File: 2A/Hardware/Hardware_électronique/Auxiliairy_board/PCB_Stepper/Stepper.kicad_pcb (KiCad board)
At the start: 2 copper layers, 35 x 30 mm, 45 parts, among them J1 UART_IN, J2 Conn_ST_STDC14, J3 Conn_01x03_Pin, J4 Conn_01x03_Pin, U4 AZ1117-3.3, U5 STM32G071CBUx

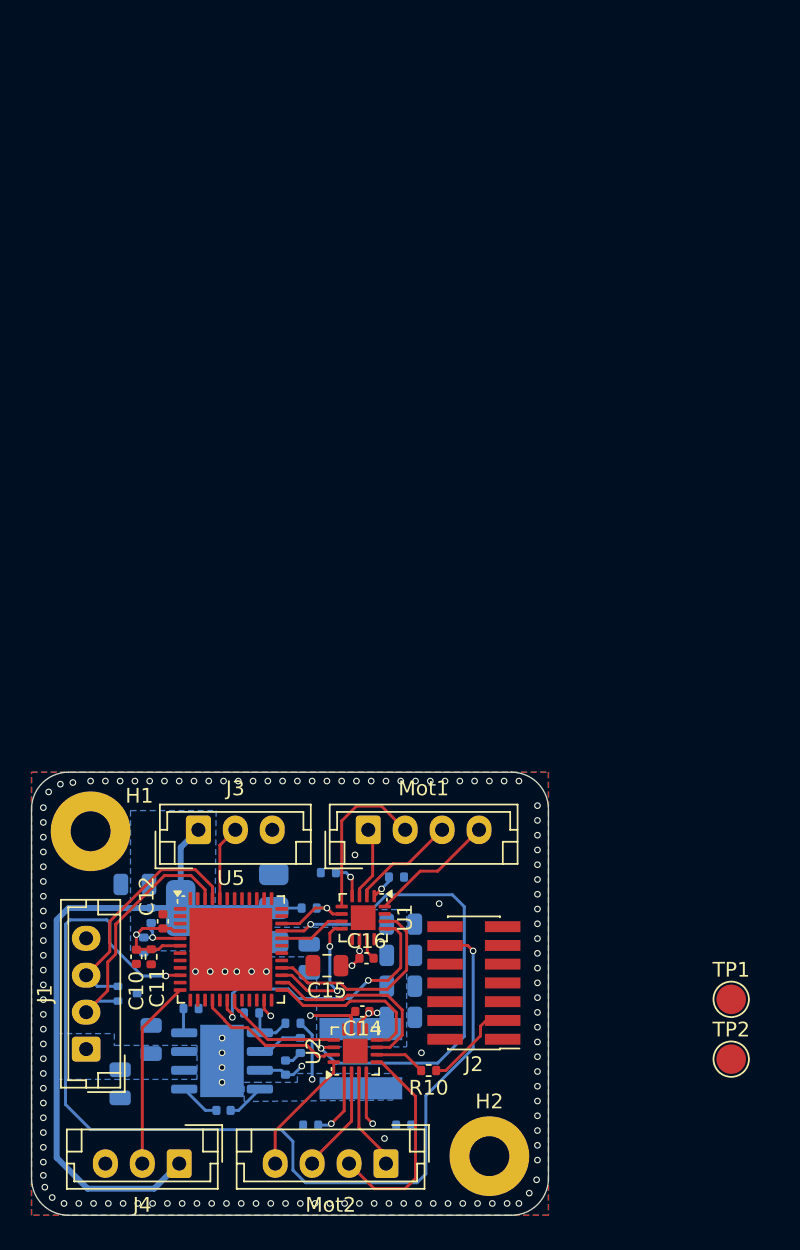
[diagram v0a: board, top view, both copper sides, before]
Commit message: recommit to be sure...
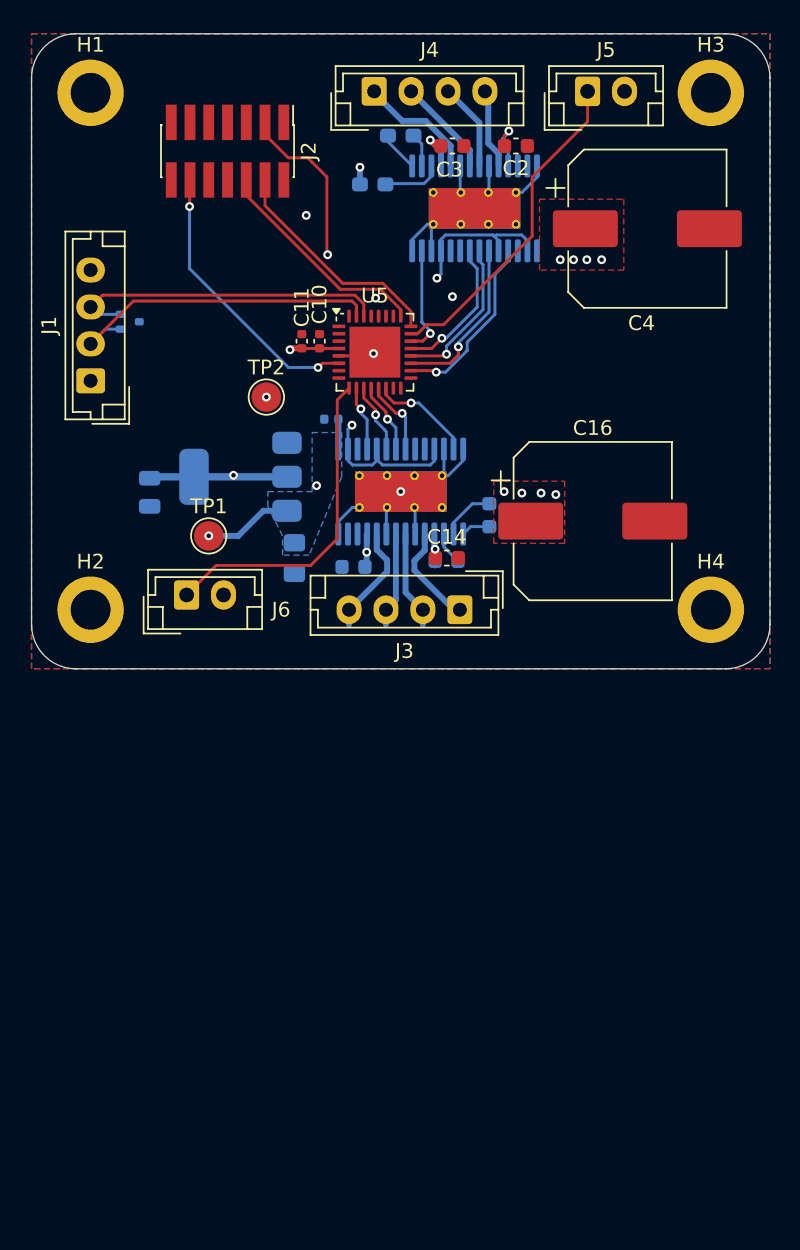
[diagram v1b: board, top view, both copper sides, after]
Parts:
- removed C5, C6, C7: 22u, Capacitor_SMD:C_0805_2012Metric
- removed L1: 15u, MainBoard:PA5432.472NLT
- removed Mot1, Mot2: Conn_01x04_Pin, Connector_JST:JST_EH_B4B-EH-A_1x04_P2.50mm_Vertical
- removed R1: 200k, Resistor_SMD:R_0402_1005Metric
- removed R10, R5: R_Small, Resistor_SMD:R_0402_1005Metric
- removed R11, R12: 10k, Resistor_SMD:R_0402_1005Metric
- removed R2: 19.6k, Resistor_SMD:R_0402_1005Metric
- removed R3: 100k, Resistor_SMD:R_0402_1005Metric
- removed R4: 11k, Resistor_SMD:R_0402_1005Metric
- removed R6, R7, R8, R9: 400m, Resistor_SMD:R_0402_1005Metric
- removed U3: ~, Package_SO:SOIC-8-1EP_3.9x4.9mm_P1.27mm_EP2.95x4.9mm_Mask2.71x3.4mm
- added C17: 22n, Capacitor_SMD:C_0603_1608Metric_Pad1.08x0.95mm_HandSolder, B.Cu at (125.0, 56.9)
- added C18: 100n, Capacitor_SMD:C_0603_1608Metric_Pad1.08x0.95mm_HandSolder, B.Cu at (123.1, 60.2)
- added H3: MountingHole_Pad, MountingHole:MountingHole_2.7mm_M2.5_ISO7380_Pad, F.Cu at (146.0, 54.0)
- added H4: MountingHole_Pad, MountingHole:MountingHole_2.7mm_M2.5_ISO7380_Pad, F.Cu at (146.0, 89.0)
- added J5: FinCourse1, Connector_JST:JST_EH_B2B-EH-A_1x02_P2.50mm_Vertical, F.Cu at (137.7, 53.9)
- added J6: FinCourse2, Connector_JST:JST_EH_B2B-EH-A_1x02_P2.50mm_Vertical, F.Cu at (110.5, 88.0)
- C1: value 10u -> 2u2; footprint Capacitor_SMD:C_0805_2012Metric -> Capacitor_SMD:C_0402_1005Metric
- C11: footprint Resistor_SMD:R_0402_1005Metric -> Capacitor_SMD:C_0402_1005Metric
- C12: value 100n -> 22n; footprint Capacitor_SMD:C_0402_1005Metric -> Capacitor_SMD:C_0603_1608Metric; moved to B.Cu
- C13: value 10u -> 100n; footprint Capacitor_SMD:C_0805_2012Metric -> Capacitor_SMD:C_0603_1608Metric
- C14: footprint Capacitor_SMD:C_0402_1005Metric -> Capacitor_SMD:C_0603_1608Metric
- C15: value 10u -> 100n; footprint Capacitor_SMD:C_0805_2012Metric -> Capacitor_SMD:C_0603_1608Metric; moved to B.Cu
- C16: value 100n -> 100u; footprint Capacitor_SMD:C_0402_1005Metric -> Capacitor_SMD:CP_Elec_10x10.5
- C2: value 10u -> 100n; footprint Capacitor_SMD:C_0805_2012Metric -> Capacitor_SMD:C_0603_1608Metric; moved to F.Cu
- C3: value 2.2n -> 100n; footprint Capacitor_SMD:C_0402_1005Metric -> Capacitor_SMD:C_0603_1608Metric; moved to F.Cu
- C4: value 100n -> 100u; footprint Capacitor_SMD:C_0402_1005Metric -> Capacitor_SMD:CP_Elec_10x10.5; moved to F.Cu
- C8: footprint Capacitor_SMD:C_0805_2012Metric -> Capacitor_SMD:C_0805_2012Metric_Pad1.18x1.45mm_HandSolder
- H1, H2: footprint MountingHole:MountingHole_2.7mm_M2.5_Pad -> MountingHole:MountingHole_2.7mm_M2.5_ISO7380_Pad
- J3, J4: value Conn_01x03_Pin -> Conn_01x04; footprint Connector_JST:JST_EH_B3B-EH-A_1x03_P2.50mm_Vertical -> Connector_JST:JST_EH_B4B-EH-A_1x04_P2.50mm_Vertical
- TP1: value TestPoint -> 5V
- TP2: value TestPoint -> 3.3V
- U1, U2: value ~ -> TMC2225; footprint Package_DFN_QFN:WQFN-16-1EP_3x3mm_P0.5mm_EP1.68x1.68mm -> Package_SO:HTSSOP-28-1EP_4.4x9.7mm_P0.65mm_EP2.75x6.2mm_ThermalVias; moved to B.Cu
- U5: value STM32G071CBUx -> STM32G071KBUx; footprint Package_DFN_QFN:QFN-48-1EP_7x7mm_P0.5mm_EP5.6x5.6mm -> Package_DFN_QFN:QFN-32-1EP_5x5mm_P0.5mm_EP3.45x3.45mm
- moved J4 73.8 mm to (123.2, 53.9), turned to 0 degrees
- moved C2 68.9 mm to (132.8, 57.6), turned to 0 degrees
- moved C4 66.2 mm to (141.7, 63.2)
- moved C3 63.4 mm to (128.5, 57.6), turned to 0 degrees
- moved J2 58.7 mm to (113.3, 58.0), turned to -90 degrees
- moved TP2 54.8 mm to (115.9, 74.6)
- moved H1 50.0 mm to (104.0, 54.0)
- moved U1 48.6 mm to (130.0, 61.8)
- moved TP1 47.3 mm to (112.0, 84.0)
- moved H2 45.8 mm to (104.0, 89.0)
- moved D1 45.5 mm to (106.7, 69.5)
- moved J1 45.3 mm to (104.0, 73.5)
- moved C1 43.7 mm to (120.3, 76.1), turned to 0 degrees
- moved C10 43.5 mm to (119.5, 70.8), turned to 90 degrees
- moved C11 42.9 mm to (118.3, 70.8), turned to 90 degrees
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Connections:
- C1 pad 1: VBUS -> GND
- C1 pad 2: GND -> +5V
- C12 pad 1: +3.3V -> Net-(U2-CPO)
- C12 pad 2: GND -> Net-(U2-CPI)
- C13 pad 1: +9V -> VBUS
- C13 pad 2: GND -> Net-(U2-VCP)
- C14 pad 1: +9V -> VBUS
- C15 pad 1: +9V -> VBUS
- C16 pad 1: +9V -> VBUS
- C3 pad 1: Net-(C3-Pad1) -> VBUS
- C4 pad 1: Net-(U3-BST) -> VBUS
- C4 pad 2: Net-(U3-SW) -> GND
- C8 pad 1: +9V -> +5V
- J3 pad 1: +3.3V -> /U2_OA2
- J3 pad 2: /SwitchL -> /U2_OA1
- J3 pad 3: GND -> /U2_OB1
- J4 pad 1: +3.3V -> /U1_OA2
- J4 pad 2: /SwitchR -> /U1_OA1
- J4 pad 3: GND -> /U1_OB1
- TP1 pad 1: +9V -> +5V
- U1 pad 10: +9V -> /U1_OB2
- U1 pad 11: GND -> VBUS
- U1 pad 12: (no net) -> unconnected-(U1-VREF-Pad12)
- U1 pad 13: //PWM1 -> unconnected-(U1-NC-Pad13)
- U1 pad 14: /PWM1 -> GND
- U1 pad 15: //sleep1 -> unconnected-(U1-5VOUT-Pad15)
- U1 pad 16: Net-(Mot1-Pin_4) -> +3.3V
- U1 pad 17: (no net) -> unconnected-(U1-PDN_UART-Pad17)
- U1 pad 4: Net-(U1-BISEN) -> VBUS
- U1 pad 5: Net-(Mot1-Pin_2) -> /U1_OA2
- U1 pad 6: /nFault1 -> GND
- U1 pad 7: /PWM3 -> /U1_OA1
- U1 pad 8: //PWM3 -> /U1_OB1
- U1 pad 9: (no net) -> GND
- U2 pad 1: Net-(U2-AISEN) -> Net-(U2-CPO)
- U2 pad 10: +9V -> /U2_OB2
- U2 pad 11: GND -> VBUS
- U2 pad 12: (no net) -> unconnected-(U2-VREF-Pad12)
- U2 pad 13: //PWM2 -> unconnected-(U2-NC-Pad13)
- U2 pad 14: /PWM2 -> GND
- U2 pad 15: //sleep2 -> +5V
- U2 pad 16: Net-(Mot2-Pin_4) -> +3.3V
- U2 pad 17: (no net) -> unconnected-(U2-PDN_UART-Pad17)
- U2 pad 2: Net-(Mot2-Pin_3) -> Net-(U2-CPI)
- U2 pad 3: Net-(Mot2-Pin_1) -> Net-(U2-VCP)
- U2 pad 4: Net-(U2-BISEN) -> VBUS
- U2 pad 5: Net-(Mot2-Pin_2) -> /U2_OA2
- U2 pad 6: /nFault2 -> GND
- U2 pad 7: /PWM4 -> /U2_OA1
- U2 pad 8: //PWM4 -> /U2_OB1
- U2 pad 9: (no net) -> GND
- U4 pad 3: +9V -> +5V
- U5 pad 10: /NRST -> /DIAG2
- U5 pad 11: unconnected-(U5-PA0-Pad11) -> /dir2
- U5 pad 12: /SwitchR -> /~{EN2}
- U5 pad 13: unconnected-(U5-PA2-Pad13) -> /step2
- U5 pad 14: unconnected-(U5-PA3-Pad14) -> /index2
- U5 pad 16: //sleep2 -> unconnected-(U5-PB1-Pad16)
- U5 pad 18: //PWM1 -> /DIAG1
- U5 pad 19: //PWM2 -> /dir1
- U5 pad 20: unconnected-(U5-PB1-Pad20) -> /~{EN1}
- U5 pad 21: unconnected-(U5-PB2-Pad21) -> /step1
- U5 pad 22: /nFault2 -> /index1
- U5 pad 23: //sleep1 -> /Course1
- U5 pad 24: unconnected-(U5-PB12-Pad24) -> /SWDIO
- U5 pad 25: //PWM4 -> /SWCLK
- U5 pad 26: /PWM4 -> unconnected-(U5-PA15-Pad26)
- U5 pad 27: //PWM3 -> unconnected-(U5-PB3-Pad27)
- U5 pad 28: /PWM1 -> unconnected-(U5-PB4-Pad28)
- U5 pad 30: unconnected-(U5-PC6-Pad30) -> /TX
- U5 pad 31: unconnected-(U5-PC7-Pad31) -> /RX
- U5 pad 32: /PWM3 -> unconnected-(U5-PB8-Pad32)
- U5 pad 33: /PWM2 -> GND
- U5 pad 5: Net-(U5-VREF+) -> GND
- U5 pad 6: +3.3V -> /NRST
- U5 pad 7: GND -> unconnected-(U5-PA0-Pad7)
- U5 pad 9: unconnected-(U5-PF1-Pad9) -> /Course2
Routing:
- net /NRST: track 69.0 -> 19.0 mm
- net /PWM2: track 34.3 -> 0.00 mm, vias 2 -> 0
- net /Course1: track 0.00 -> 22.3 mm
- net /Course2: track 0.00 -> 22.3 mm
- net //PWM1: track 19.1 -> 0.00 mm, vias 2 -> 0
- net +3.3V: track 62.2 -> 46.0 mm, vias 1 -> 6
- net /SWDIO: track 0.00 -> 15.6 mm
- net /SWCLK: track 0.00 -> 15.2 mm
- net GND: track 9.32 -> 24.1 mm, vias 136 -> 7
- net Net-(Mot2-Pin_2): track 14.6 -> 0.00 mm
- net /PWM1: track 14.0 -> 0.00 mm
- net /PWM4: track 12.9 -> 0.00 mm
- net /SwitchR: track 12.8 -> 0.00 mm
- net /DIAG1: track 0.00 -> 12.4 mm, vias 0 -> 1
- net VBUS: track 0.00 -> 12.3 mm, vias 0 -> 12
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- added copper zone on In2.Cu, net +3.3V
- added copper zone on B.Cu, net +5V
- added copper zone on In1.Cu, net GND
- added copper zone on F.Cu, net VBUS
- added copper zone on In2.Cu, net VBUS
- removed copper zone on B.Cu, net +3.3V
- removed copper zone on B.Cu, net +9V
- removed copper zone on B.Cu, net Net-(U3-SW)
- removed copper zone on B.Cu, net VBUS
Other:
- board size 35 x 30 mm -> 50 x 43 mm
- copper layers 2 -> 4
